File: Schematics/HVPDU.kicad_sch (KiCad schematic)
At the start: 32 parts, among them J35 BAMOCAR, J36 MCU CAN, J37 MCU COM, J38 3-2325013-1, J39 Energy Meter Current, J40 PL00X-301-10M8, J41 PL00Y-301-10M8, J42 HVD, J43 MCU Resolver, J44 Energy Meter Voltage, J45 Energy meter COM port, J46 DCDC HV side, J47 DCDC LV Side, J48 CCCV IN, J49 CCCV OUT, J50 RT00122PNH03, J51 TSAL_R, J52 TSMP+, J53 TSMP-, J54 GLVMP, J55 DT04-3P-L012, J56 DT04-4P-L012, J57 DHAB S/106, J58 12V power plug, J59 GND PLUG, J60 DT04-6P-L012, J61 DT04-8P-L012, J62 RT00104PN03, J63 RT00104PN03, J65 HD10-9-1939P, K6 DISCHARGE RELAY GIGAVAC PNC11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

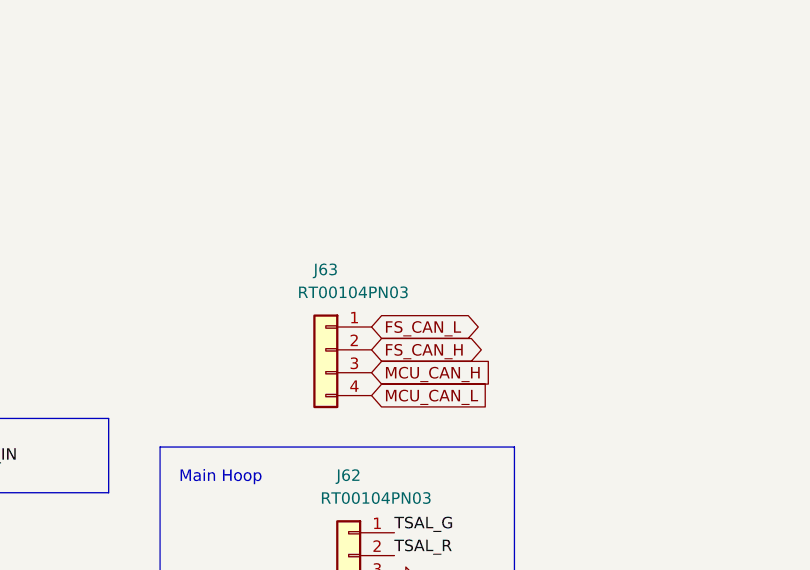
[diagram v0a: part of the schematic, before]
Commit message: push stuffs
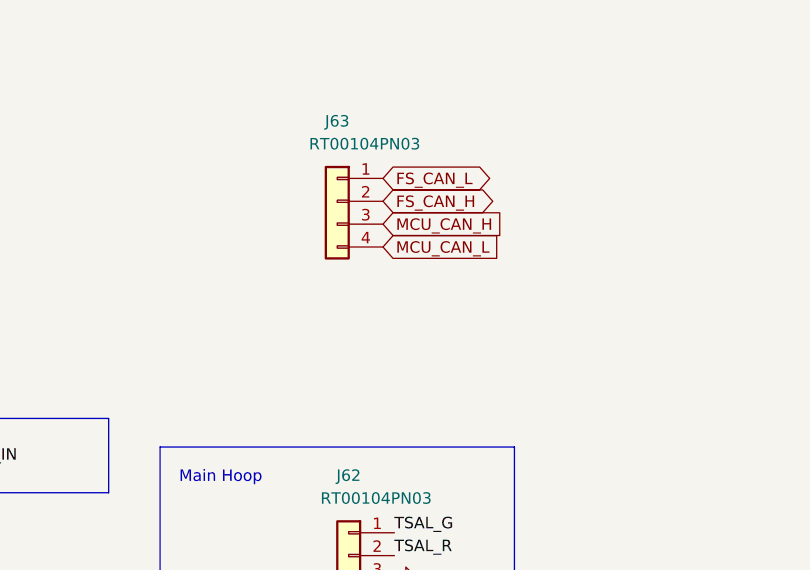
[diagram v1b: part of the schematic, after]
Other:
- moved on the sheet: J63
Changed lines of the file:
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@@
 	(global_label "FS_CAN_L"
 		(shape bidirectional)
-		(at 353.06 39.37 0)
-		(fields_autoplaced yes)
-		(effects
-			(font
-				(size 1.27 1.27)
-			)
-			(justify left)
-		)
-		(property "Intersheetrefs" "${INTERSHEET_REFS}"
-			(at 366.107 39.37 0)
+		(at 354.33 22.86 0)
+		(fields_autoplaced yes)
+		(effects
+			(font
+				(size 1.27 1.27)
+			)
+			(justify left)
+		)
+		(property "Intersheetrefs" "${INTERSHEET_REFS}"
+			(at 367.377 22.86 0)
 			(hide yes)
 			(show_name no)
@@
 	(global_label "MCU_CAN_L"
 		(shape input)
-		(at 353.06 46.99 0)
-		(fields_autoplaced yes)
-		(effects
-			(font
-				(size 1.27 1.27)
-			)
-			(justify left)
-		)
-		(property "Intersheetrefs" "${INTERSHEET_REFS}"
-			(at 366.7495 46.99 0)
+		(at 354.33 30.48 0)
+		(fields_autoplaced yes)
+		(effects
+			(font
+				(size 1.27 1.27)
+			)
+			(justify left)
+		)
+		(property "Intersheetrefs" "${INTERSHEET_REFS}"
+			(at 368.0195 30.48 0)
 			(hide yes)
 			(show_name no)
@@
 	(global_label "FS_CAN_H"
 		(shape bidirectional)
-		(at 353.06 41.91 0)
-		(fields_autoplaced yes)
-		(effects
-			(font
-				(size 1.27 1.27)
-			)
-			(justify left)
-		)
-		(property "Intersheetrefs" "${INTERSHEET_REFS}"
-			(at 366.4094 41.91 0)
+		(at 354.33 25.4 0)
+		(fields_autoplaced yes)
+		(effects
+			(font
+				(size 1.27 1.27)
+			)
+			(justify left)
+		)
+		(property "Intersheetrefs" "${INTERSHEET_REFS}"
+			(at 367.6794 25.4 0)
 			(hide yes)
 			(show_name no)
@@
 	(global_label "MCU_CAN_H"
 		(shape input)
-		(at 353.06 44.45 0)
-		(fields_autoplaced yes)
-		(effects
-			(font
-				(size 1.27 1.27)
-			)
-			(justify left)
-		)
-		(property "Intersheetrefs" "${INTERSHEET_REFS}"
-			(at 367.0519 44.45 0)
+		(at 354.33 27.94 0)
+		(fields_autoplaced yes)
+		(effects
+			(font
+				(size 1.27 1.27)
+			)
+			(justify left)
+		)
+		(property "Intersheetrefs" "${INTERSHEET_REFS}"
+			(at 368.3219 27.94 0)
 			(hide yes)
 			(show_name no)
@@
 	(symbol
 		(lib_id "Connector_Generic:Conn_01x04")
-		(at 347.98 41.91 0)
+		(at 349.25 25.4 0)
 		(mirror y)
 		(unit 1)
@@
 		(dnp no)
 		(property "Reference" "J63"
-			(at 347.98 33.02 0)
+			(at 349.25 16.51 0)
 			(show_name no)
 			(do_not_autoplace no)
@@
 		)
 		(property "Value" "RT00104PN03"
-			(at 351.028 35.56 0)
+			(at 352.298 19.05 0)
 			(show_name no)
 			(do_not_autoplace no)
@@
 		)
 		(property "Footprint" ""
-			(at 347.98 41.91 0)
+			(at 349.25 25.4 0)
 			(hide yes)
 			(show_name no)
@@
 		)
 		(property "Datasheet" ""
-			(at 347.98 41.91 0)
+			(at 349.25 25.4 0)
 			(hide yes)
 			(show_name no)
@@
 		)
 		(property "Description" "Generic connector, single row, 01x04, script generated (kicad-library-utils/schlib/autogen/connector/)"
-			(at 347.98 41.91 0)
-			(hide yes)
-			(show_name no)
+			(at 349.25 25.4 0)
+			(hide yes)
+			(show_name no)
